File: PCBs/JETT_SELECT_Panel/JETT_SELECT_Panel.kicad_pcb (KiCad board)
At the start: 2 copper layers, 36.3 x 99.1 mm, 36 parts, among them J1 BackLight, J2 SwithCol, J3 SwitchRow, J4 LedCathode, J5 LedAnode, P3 CONN_01X01, P4 CONN_01X01, SW1 SW_Push, SW2 SW_Push, SW3 SW_Push, SW4 SW_Push, SW5 SW_Push

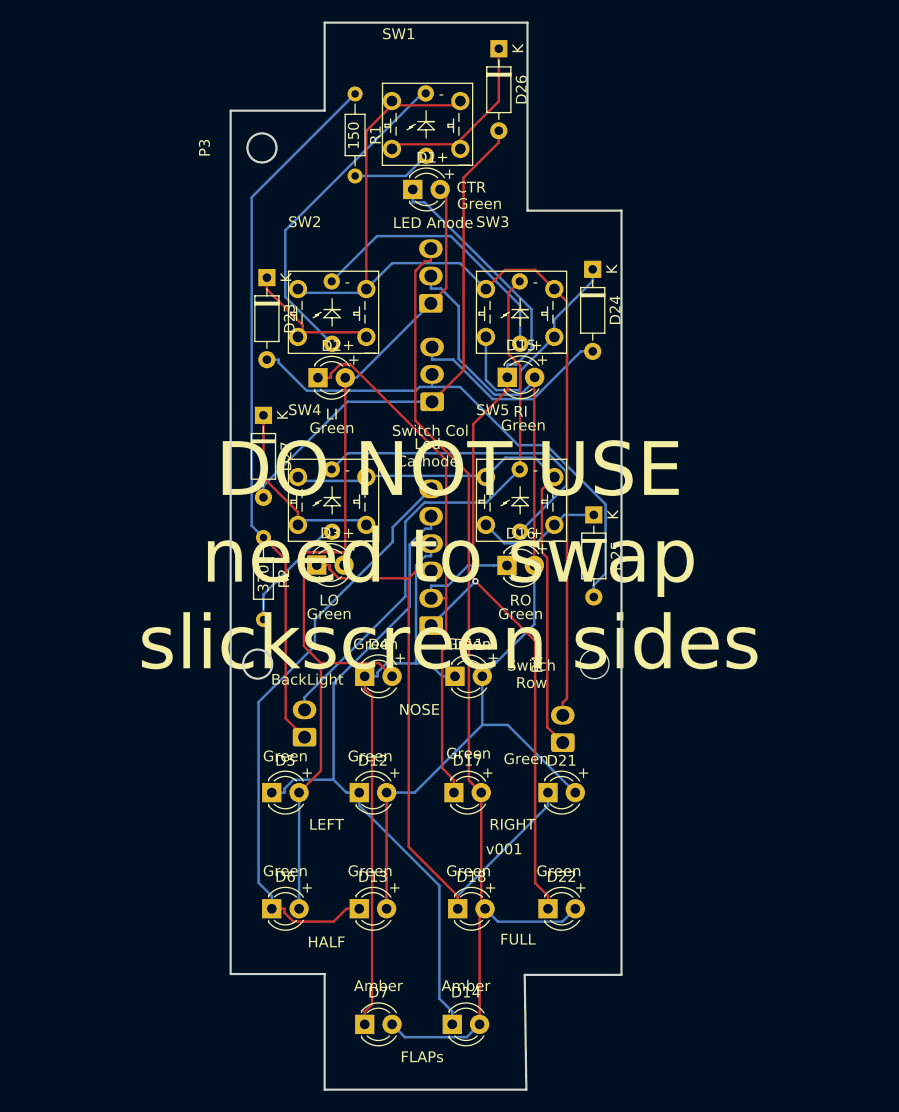
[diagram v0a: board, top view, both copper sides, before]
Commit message: PCB
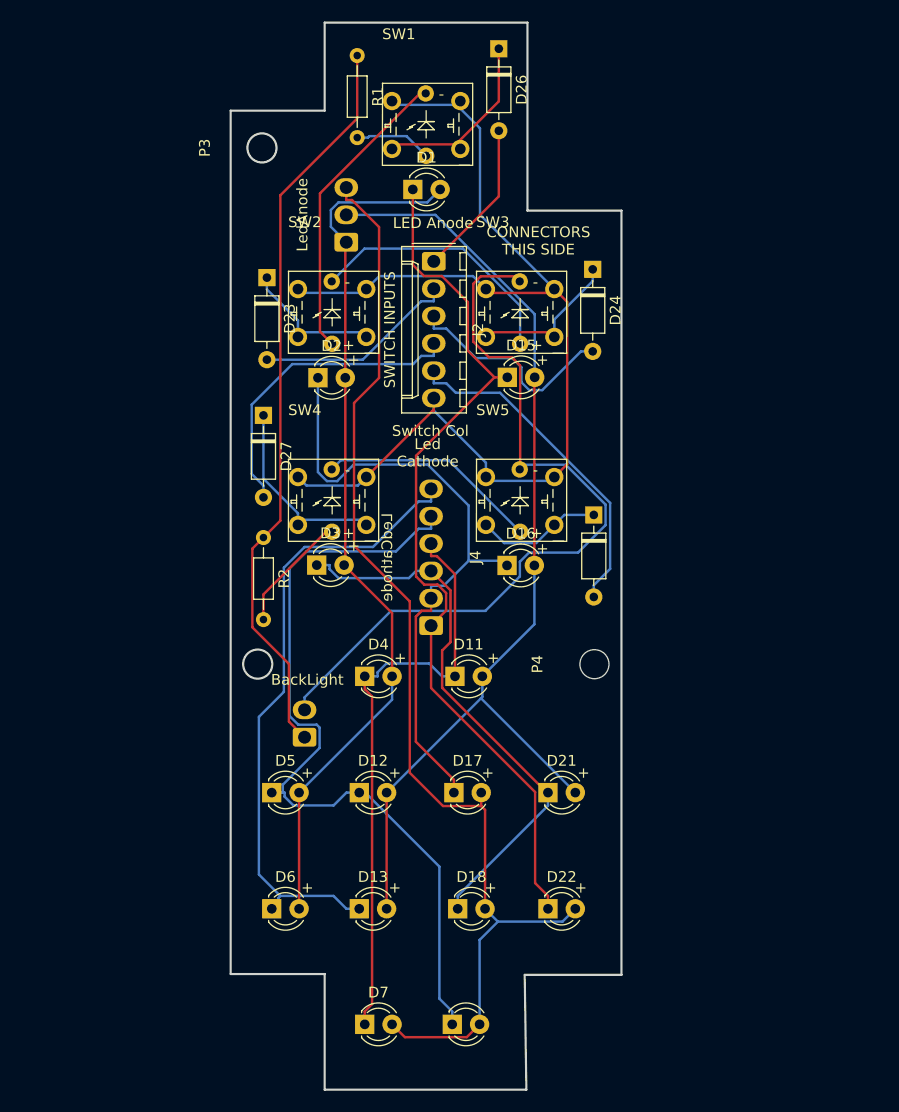
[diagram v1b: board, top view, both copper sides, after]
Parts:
- removed J3: SwitchRow, PT_Library_v001:Molex_1x02_P2.54mm_Vertical
- J2: value SwithCol -> SWITCH INPUTS; footprint PT_Library_v001:Molex_1x03_P2.54mm_Vertical -> PT_Library_v001:Molex_1x06_P2.54mm_Vertical; moved to F.Cu
- moved J2 13.0 mm to (103.2, 69.5), turned to 270 degrees
- moved J5 9.70 mm to (95.1, 67.7)
- moved R1 3.57 mm to (96.1, 50.4)
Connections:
- net Net-(D24-Pad2) renamed /COL8
- D23 pad 2: Net-(D23-Pad2) -> /COL7
- D25 pad 2: Net-(D23-Pad2) -> /COL10
- D26 pad 2: Net-(D26-Pad2) -> /COL6
- D27 pad 2: Net-(D26-Pad2) -> /COL9
- J2 pad 1: Net-(D26-Pad2) -> /COL6
- J2 pad 2: Net-(D23-Pad2) -> /COL7
- SW1 pad 3: Net-(J3-Pad2) -> /ROW15
- SW1 pad 4: Net-(J3-Pad2) -> /ROW15
- SW2 pad 3: Net-(J3-Pad2) -> /ROW15
- SW2 pad 4: Net-(J3-Pad2) -> /ROW15
- SW3 pad 3: Net-(J3-Pad2) -> /ROW15
- SW3 pad 4: Net-(J3-Pad2) -> /ROW15
- SW4 pad 3: Net-(J3-Pad1) -> /ROW15
- SW4 pad 4: Net-(J3-Pad1) -> /ROW15
- SW5 pad 3: Net-(J3-Pad1) -> /ROW15
- SW5 pad 4: Net-(J3-Pad1) -> /ROW15
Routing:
- net /ROW15: track 0.00 -> 104.3 mm
- net Net-(J3-Pad2): track 92.8 -> 0.00 mm
- net Net-(J3-Pad1): track 51.6 -> 0.00 mm
- net Net-(D26-Pad2): track 47.7 -> 0.00 mm
- net Net-(D23-Pad2): track 47.7 -> 0.00 mm
- net /COL10: track 0.00 -> 31.5 mm
- net /COL9: track 0.00 -> 29.0 mm
- net Net-(J1-Pad2): track 52.3 -> 73.2 mm
- net /COL7: track 0.00 -> 18.9 mm
- net /COL6: track 0.00 -> 14.6 mm
- net /SegB: track 94.3 -> 106.6 mm
- net /Dig4: track 63.0 -> 75.0 mm
- net Net-(SW4-Pad6): track 30.5 -> 20.6 mm
- net /SegA: track 86.4 -> 94.6 mm
- net Net-(D24-Pad1): track 21.5 -> 14.5 mm
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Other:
- board text added: "COMPONENTS THIS SIDE"
- board text added: "CONNECTORS THIS SIDE"
- board text added: "V002"
- board text removed: "DO NOT USE need to swap slickscreen sides"
- board text removed: "Switch Row"
- board text removed: "v001"
